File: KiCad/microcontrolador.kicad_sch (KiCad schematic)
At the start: 20 parts, among them J2 DE9_Pins_MountingHoles, J3 Conn_01x05, J5 DE9_Pins_MountingHoles, U4 MCP2551-I-SN, U7 PIC24HJ128GP502, Y1 8MHz

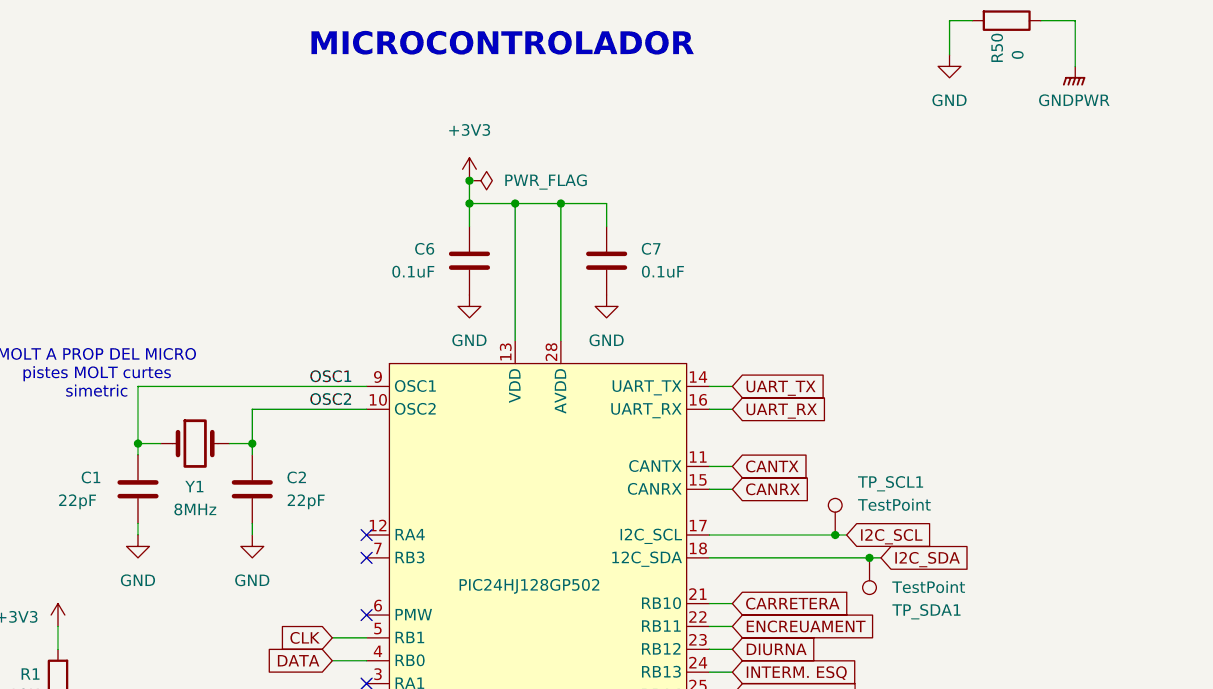
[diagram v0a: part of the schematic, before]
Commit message: test points schematic
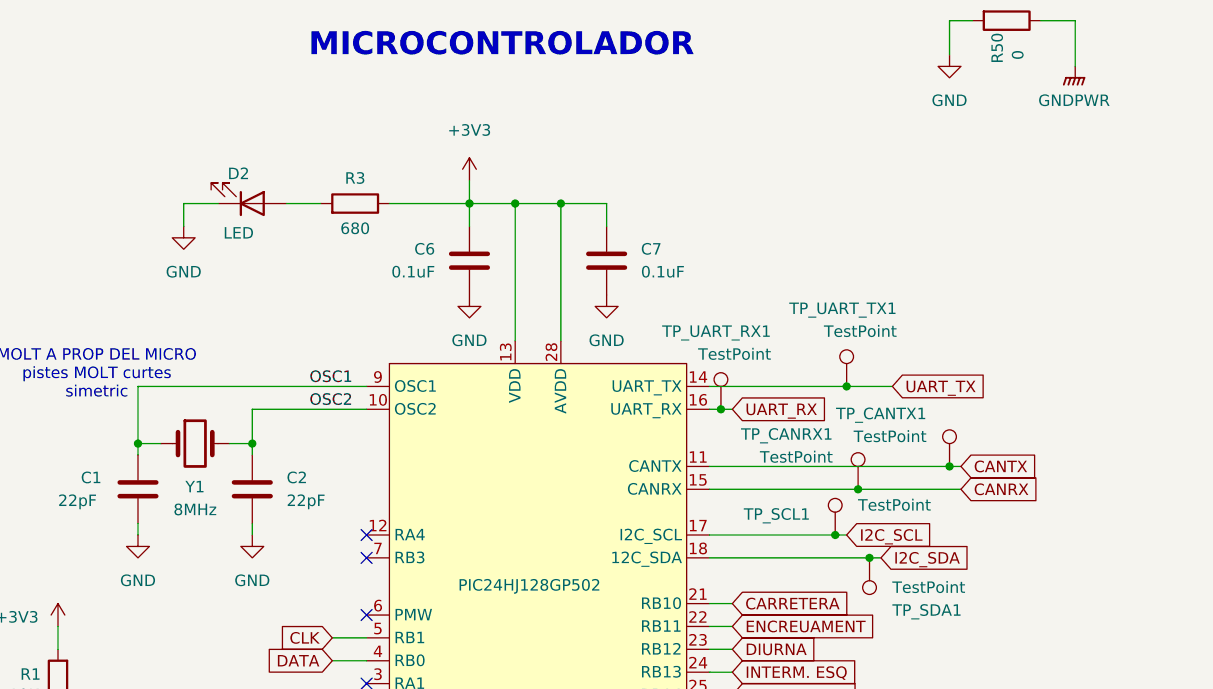
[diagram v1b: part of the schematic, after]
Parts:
- added D2: LED, LED_SMD:LED_0805_2012Metric_Pad1.15x1.40mm_HandSolder, symbol Device:LED
- added R3: 680, Resistor_SMD:R_0805_2012Metric_Pad1.20x1.40mm_HandSolder, symbol Device:R
- added TP_CANRX1, TP_CANTX1, TP_UART_RX1, TP_UART_TX1: TestPoint, Connector_PinHeader_2.54mm:PinHeader_1x01_P2.54mm_Vertical, symbol Connector:TestPoint
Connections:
- net +3V3: now also R3.1
- net CANRX: now also TP_CANRX1.1
- net CANTX: now also TP_CANTX1.1
- net GND: now also D2.1 (K)
- net UART_RX: now also TP_UART_RX1.1
- net UART_TX: now also TP_UART_TX1.1
- new net: D2.2 (A), R3.2

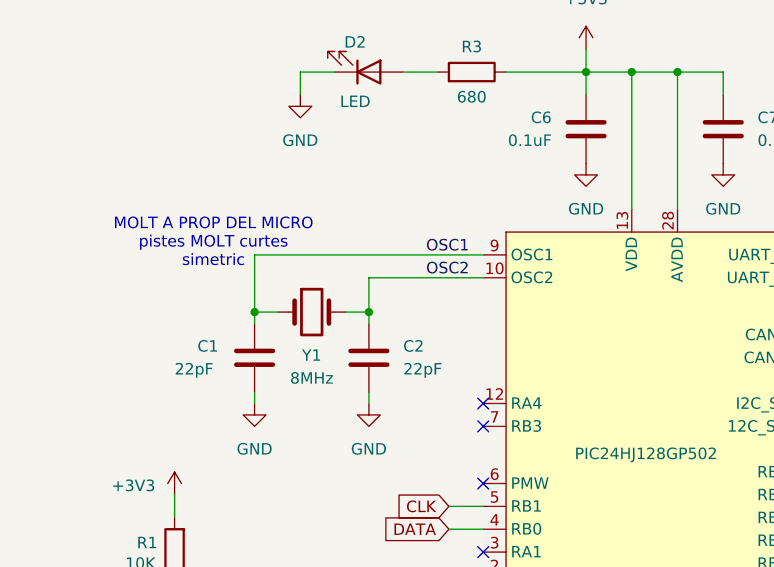
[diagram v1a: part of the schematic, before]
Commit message: errors CADLAB
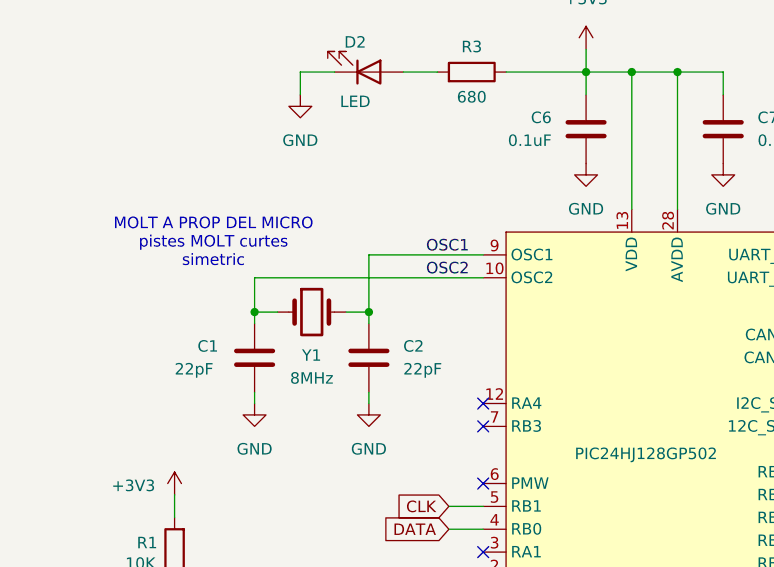
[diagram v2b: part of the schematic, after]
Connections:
- net OSC1: now also C2.1, Y1.2; no longer C1.1, Y1.1
- net OSC2: now also C1.1, Y1.1; no longer C2.1, Y1.2
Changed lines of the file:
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@@
 	(wire
 		(pts
-			(xy 77.47 76.2) (xy 90.17 76.2)
+			(xy 77.47 73.66) (xy 90.17 73.66)
 		)
 		(stroke
@@
 	(wire
 		(pts
-			(xy 77.47 80.01) (xy 77.47 76.2)
+			(xy 77.47 80.01) (xy 77.47 73.66)
 		)
 		(stroke
@@
 	(wire
 		(pts
-			(xy 64.77 73.66) (xy 90.17 73.66)
+			(xy 64.77 76.2) (xy 90.17 76.2)
 		)
 		(stroke
@@
 	(wire
 		(pts
-			(xy 64.77 73.66) (xy 64.77 80.01)
+			(xy 64.77 76.2) (xy 64.77 80.01)
 		)
 		(stroke
@@
 		)
 	)
-	(label "OSC1"
-		(at 83.82 73.66 0)
+	(label "OSC2"
+		(at 83.82 76.2 0)
 		(effects
 			(font
@@
 		)
 	)
-	(label "OSC2"
-		(at 83.82 76.2 0)
+	(label "OSC1"
+		(at 83.82 73.66 0)
 		(effects
 			(font

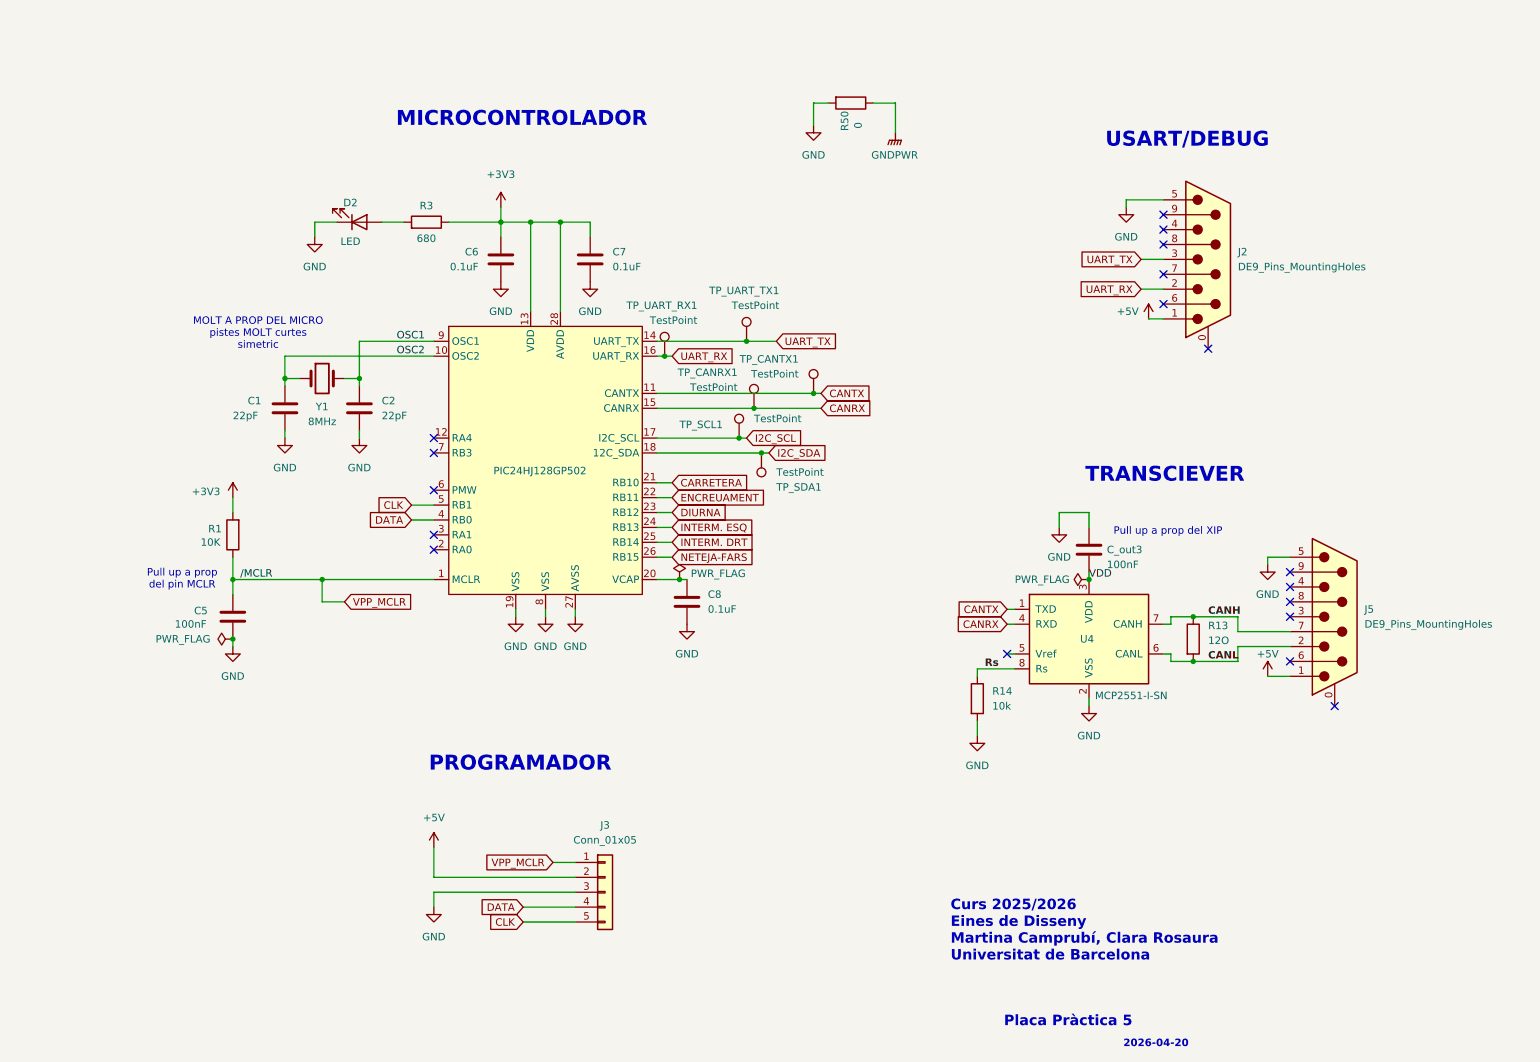
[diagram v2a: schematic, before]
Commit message: push final (?)
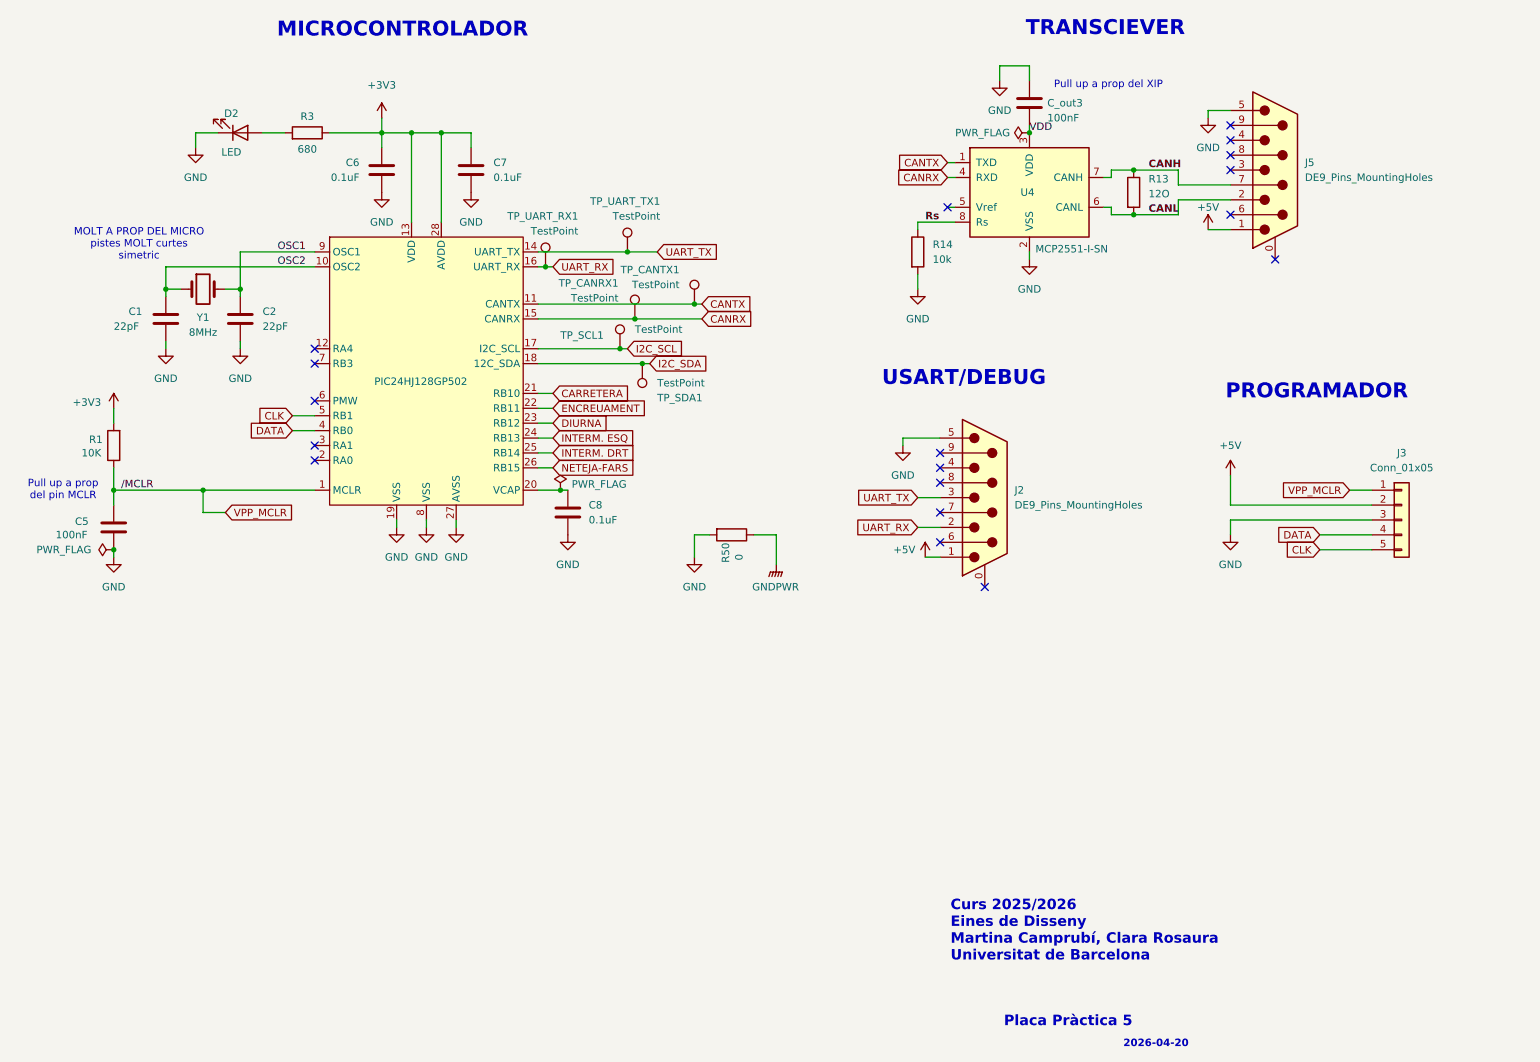
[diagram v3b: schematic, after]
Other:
- moved on the sheet: C1, C2, C5, C6, C7, C8, C_out3, D2, J2, J3, J5, R1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
